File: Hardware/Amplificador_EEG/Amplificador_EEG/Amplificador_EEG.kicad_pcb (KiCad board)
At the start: 2 copper layers, 48.4 x 59.1 mm, 50 parts, among them J1 IN, J2 REF, J3 GND, J4 POWER, J5 OUTPUT, J6 Mounting Hole, U1 LM358, U2 AD620, U3 LM358, U4 LM358, U5 LM358, U6 LM358

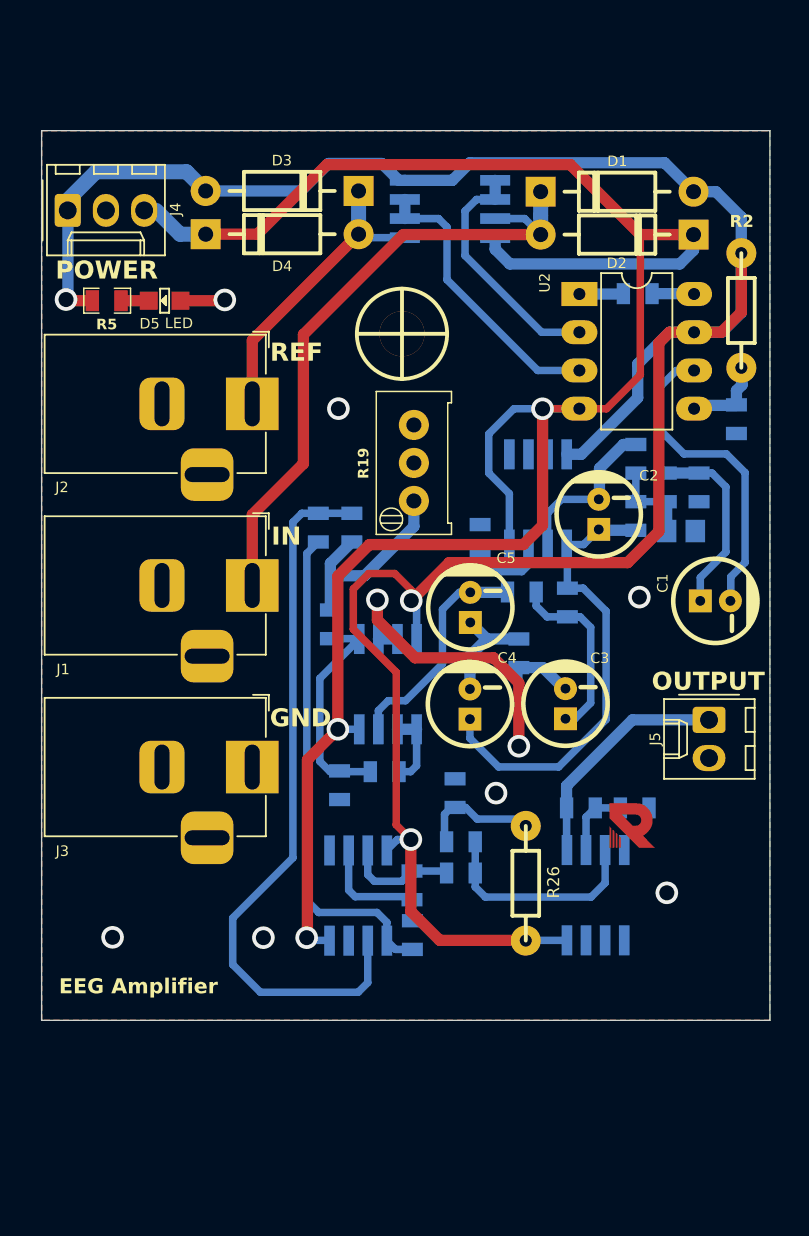
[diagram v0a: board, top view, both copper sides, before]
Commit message: Actual
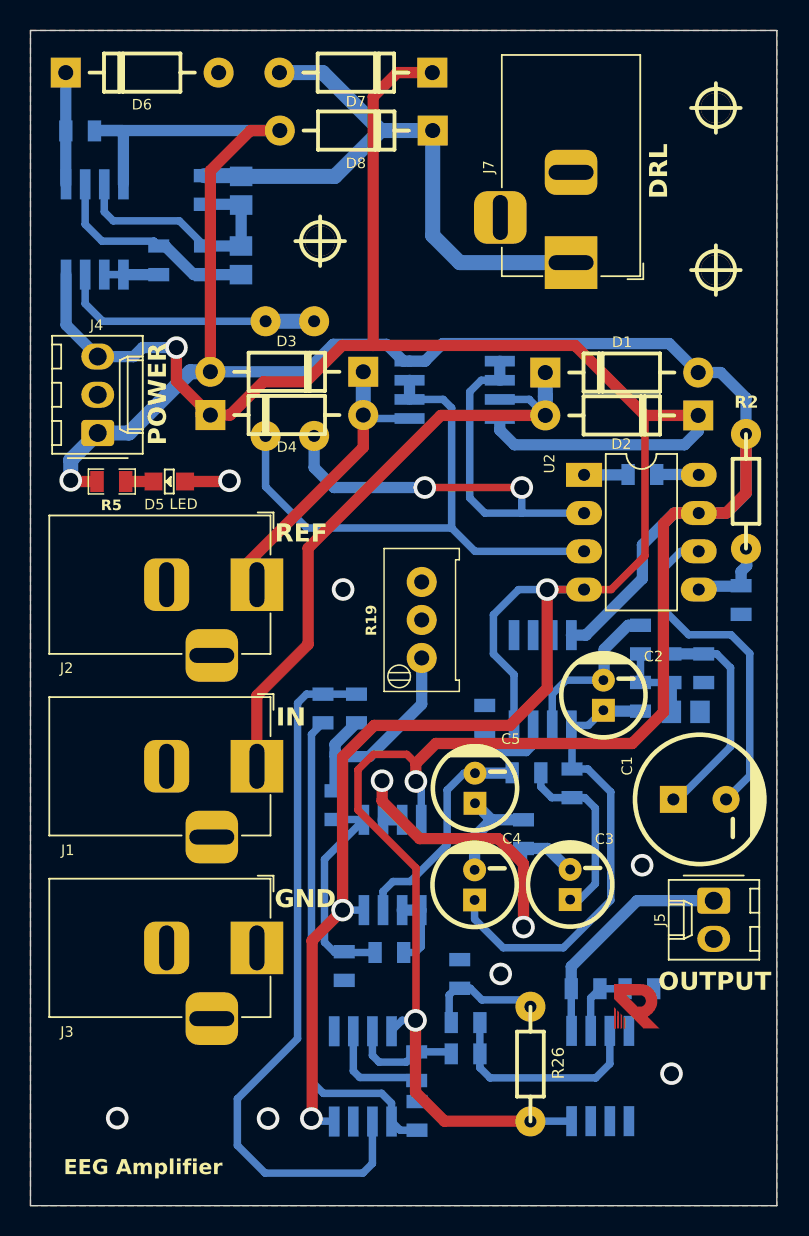
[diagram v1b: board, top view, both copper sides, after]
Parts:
- added C7: 1n, EESTN5:C_0805, B.Cu at (142.6, 76.1)
- added C8: 1n, EESTN5:C_0805, B.Cu at (142.6, 71.5)
- added D6: C2v2, EESTN5:DO-41, F.Cu at (136.0, 63.7)
- added D7: 1N4007, EESTN5:DO-41, F.Cu at (150.2, 63.7)
- added D8: 1N4007, EESTN5:DO-41, F.Cu at (150.2, 67.5)
- added J7: DRL, Connector_BarrelJack:BarrelJack_Horizontal, F.Cu at (164.5, 76.3)
- added J8: Jail Hole, EESTN5:hole_2mm, F.Cu at (174.1, 66.0)
- added J9: Jail Hole, EESTN5:hole_2mm, F.Cu at (174.1, 76.8)
- added R10: 1M, EESTN5:RES0.3, B.Cu at (144.2, 84.0)
- added R15: 10k, EESTN5:R_0805, B.Cu at (137.1, 76.1)
- added R30: 330, EESTN5:R_0805, B.Cu at (131.9, 67.5)
- added R31: 100k, EESTN5:R_0805, B.Cu at (140.1, 76.1)
- added R32: 100k, EESTN5:R_0805, B.Cu at (140.1, 71.5)
- added R8: 1M, EESTN5:RES0.3, B.Cu at (147.4, 84.0)
- added U7: LM358, EESTN5:SSOP-8, B.Cu at (132.9, 74.1)
- C1: footprint EESTN5:CAP_ELEC_5x11mm -> EESTN5:CAP_ELEC_8x11.5mm
- J6: footprint EESTN5:hole_3mm -> EESTN5:hole_2mm
- moved J4 14.9 mm to (133.1, 87.6), turned to 90 degrees
- moved C1 13.2 mm to (173.1, 112.0)
- moved C4 12.0 mm to (158.1, 117.7)
- moved C6 12.0 mm to (172.1, 106.2)
- moved J3 12.0 mm to (143.6, 121.8)
- moved R12 12.0 mm to (164.6, 110.9)
- moved R14 12.0 mm to (161.3, 114.3)
- moved R2 12.0 mm to (176.1, 91.5)
- moved R9 12.0 mm to (169.1, 105.2)
- moved U2 12.0 mm to (165.4, 90.4)
- moved C2 12.0 mm to (166.7, 105.0)
- moved C3 12.0 mm to (164.4, 117.6)
- moved C5 12.0 mm to (158.1, 111.2)
- moved D1 12.0 mm to (167.9, 86.5)
- moved D2 12.0 mm to (167.9, 83.6)
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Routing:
- net /DRL_OUT: track 0.00 -> 41.7 mm
- net -5V: track 138.1 -> 171.7 mm, vias 3 -> 4
- net +5V: track 170.1 -> 202.6 mm
- net /IN+: track 16.3 -> 36.8 mm, vias 0 -> 2
- net /IN-: track 19.1 -> 38.6 mm
- net /DRL_IN: track 0.00 -> 17.6 mm
- net Net-(U7-Out2): track 0.00 -> 17.0 mm
- net Net-(U7-IN2-): track 0.00 -> 14.4 mm
- net /DRL_REF: track 0.00 -> 7.43 mm
- net Net-(U7-IN1-): track 0.00 -> 3.22 mm
- net Net-(C1-Pad1): track 12.6 -> 14.8 mm
- net Net-(R18-Pad2): track 14.0 -> 15.7 mm
- net /AD620_OUT: track 21.4 -> 22.8 mm
- net /INPUT: track 43.1 -> 41.8 mm
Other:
- board size 48.4 x 59.1 mm -> 49.6 x 78.1 mm
